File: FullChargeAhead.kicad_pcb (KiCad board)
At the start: 2 copper layers, 18 parts, among them P101 CONN_2, P102 CONN_2, P103 MICROUSB-B, U101 MCP73834-FCI/UN

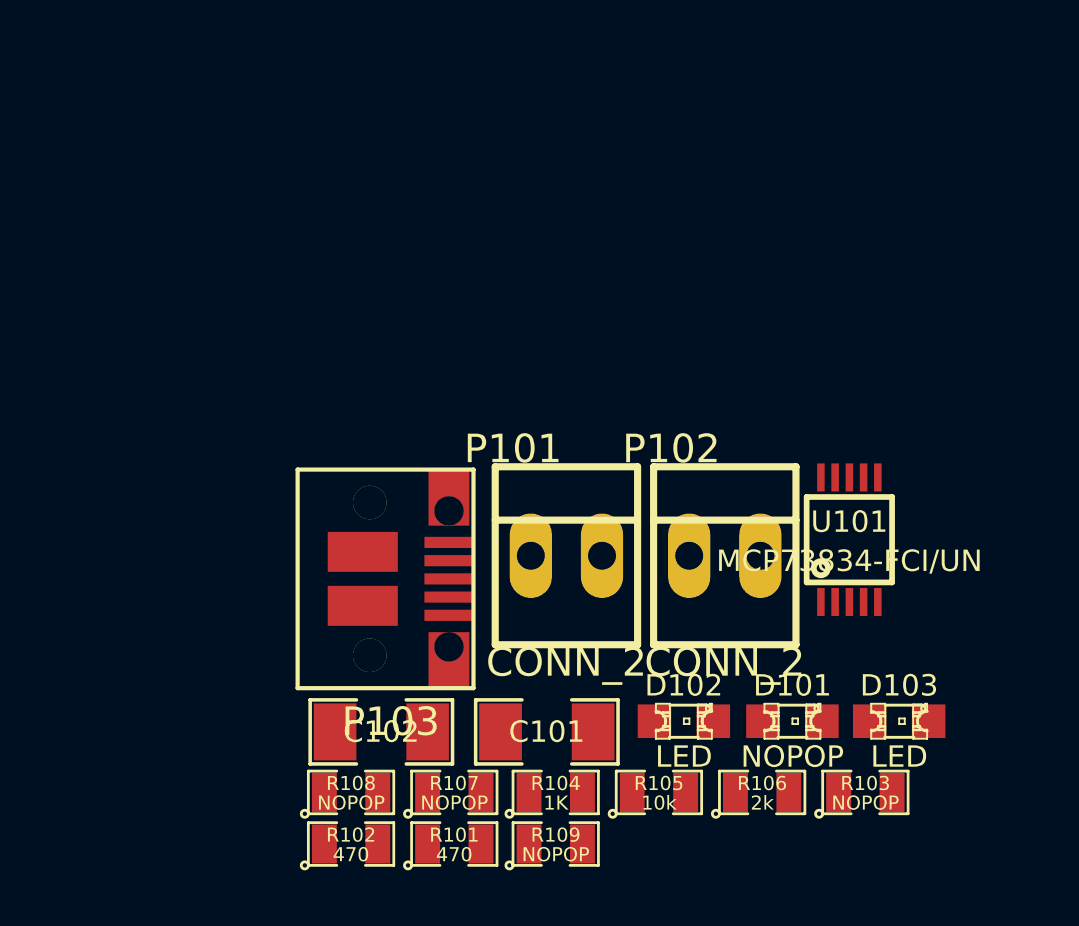
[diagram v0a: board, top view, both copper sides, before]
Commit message: Seguimos con el layout
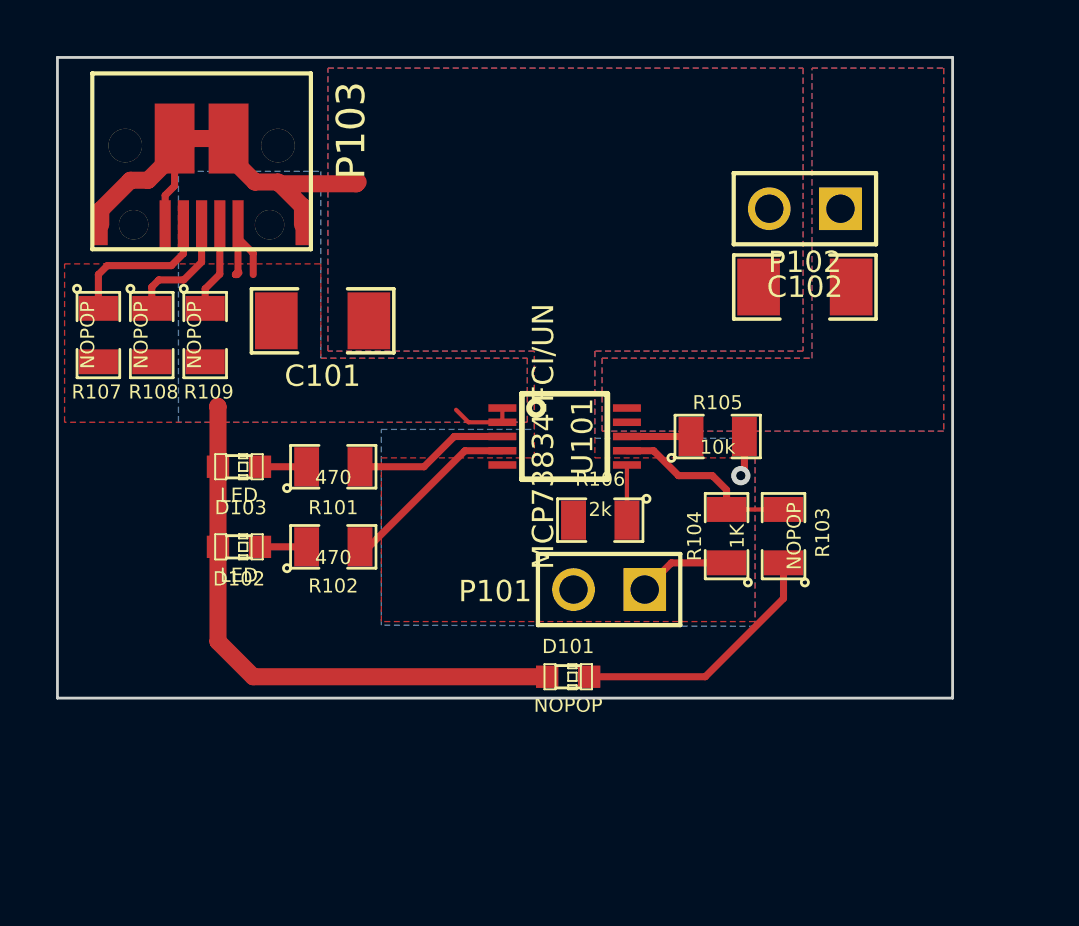
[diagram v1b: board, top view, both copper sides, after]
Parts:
- D101, D102, D103: footprint LED-0805 -> LED-0603
- P101, P102: footprint PINHEAD1-2 -> PIN_ARRAY_2X1
- P103: footprint USB_MICRO_B(10103594) -> USB_MICRO_B(10103594)v2
- moved D103 25.2 mm to (111.0, 80.8)
- moved R109 22.1 mm to (109.8, 76.1), turned to 270 degrees
- moved C102 21.9 mm to (131.2, 74.4), turned to 180 degrees
- moved R107 20.7 mm to (106.0, 76.1), turned to 270 degrees
- moved R108 17.8 mm to (107.9, 76.1), turned to 270 degrees
- moved D102 17.1 mm to (111.0, 83.7)
- moved C101 16.7 mm to (114.0, 75.6)
- moved P103 15.4 mm to (109.7, 72.2), turned to 270 degrees
- moved R101 14.1 mm to (114.4, 80.8)
- moved R105 12.9 mm to (128.1, 79.8)
- moved P102 12.7 mm to (131.2, 71.6), turned to 180 degrees
- moved R106 11.3 mm to (123.9, 82.7), turned to 180 degrees
- moved R104 11.0 mm to (128.4, 83.3), turned to 90 degrees
- moved U101 10.8 mm to (122.6, 79.8), turned to 270 degrees
- moved R102 10.6 mm to (114.4, 83.7)
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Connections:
- net N-0000014 renamed /Vdd
- net N-0000015 renamed /Vbat
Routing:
- net /Vdd: track 0.00 -> 27.1 mm
- net GND: track 0.00 -> 18.6 mm, vias 0 -> 1
- net N-000009: track 0.00 -> 9.36 mm
- net N-000004: track 0.00 -> 6.87 mm
- net N-000008: track 0.00 -> 6.50 mm
- net N-000005: track 0.00 -> 5.58 mm
- net N-0000010: track 0.00 -> 5.53 mm
- net N-000007: track 0.00 -> 4.24 mm
- net N-000001: track 0.00 -> 3.32 mm
- net N-000006: track 0.00 -> 3.20 mm
- net N-000003: track 0.00 -> 2.29 mm
- net N-0000011: track 0.00 -> 1.97 mm
- net N-0000013: track 0.00 -> 1.66 mm
- net N-0000012: track 0.00 -> 1.66 mm
- added copper zone on B.Cu, net /Vbat
- added copper zone on F.Cu, net /Vbat
- added copper zone on B.Cu, net /Vdd
- added copper zone on F.Cu, net /Vdd
- added copper zone on B.Cu, net GND
- added copper zone on F.Cu, net GND
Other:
- board outline added: 31.9 x 22.9 mm
- net class Default: clearance 0.254 -> 0.1524; trace_width 0.254 -> 0.1524; via_dia 0.889 -> 0.6858; via_drill 0.635 -> 0.3302
- rule trace_clearance: 0.254 -> 0.1524
- rule trace_min: 0.254 -> 0.1524
- rule via_min_drill: 0.508 -> 0.3302
- rule via_min_size: 0.889 -> 0.6858
